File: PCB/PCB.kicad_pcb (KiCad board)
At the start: 2 copper layers, 121.6 x 80 mm, 109 parts, among them J2 Conn, J3 Screw_Terminal_01x02, J4 Screw_Terminal_01x02, J5 Screw_Terminal_01x02, J6 Screw_Terminal_01x02, Q1 Q_NPN_BCE, Q10 Q_NPN, Q11 Q_PNP_BCE, Q12 Q_NPN, Q13 Q_PNP, Q14 Q_PNP_BCE, Q15 Q_PNP_BCE, Q16 Q-NPN, Q17 Q-NPN, Q18 Q-NPN, Q19 Q-PNP, Q2 Q_PNP_BCE, Q20 Q-NPN, Q21 Q-PNP, Q22 Q-NPN, Q23 Q-PNP, Q24 Q-PNP, Q25 Q-NPN, Q26 Q-NPN, Q27 Q-PNP, Q28 Q-NPN, Q29 Q_PNP, Q3 Q_NPN_BCE, Q4 Q_PNP_BCE, Q5 Q_NPN_BCE, Q6 Q_PNP_BCE, Q7 Q_PNP_BCE, Q8 Q_NPN_BCE, Q9 Q_NPN_BCE

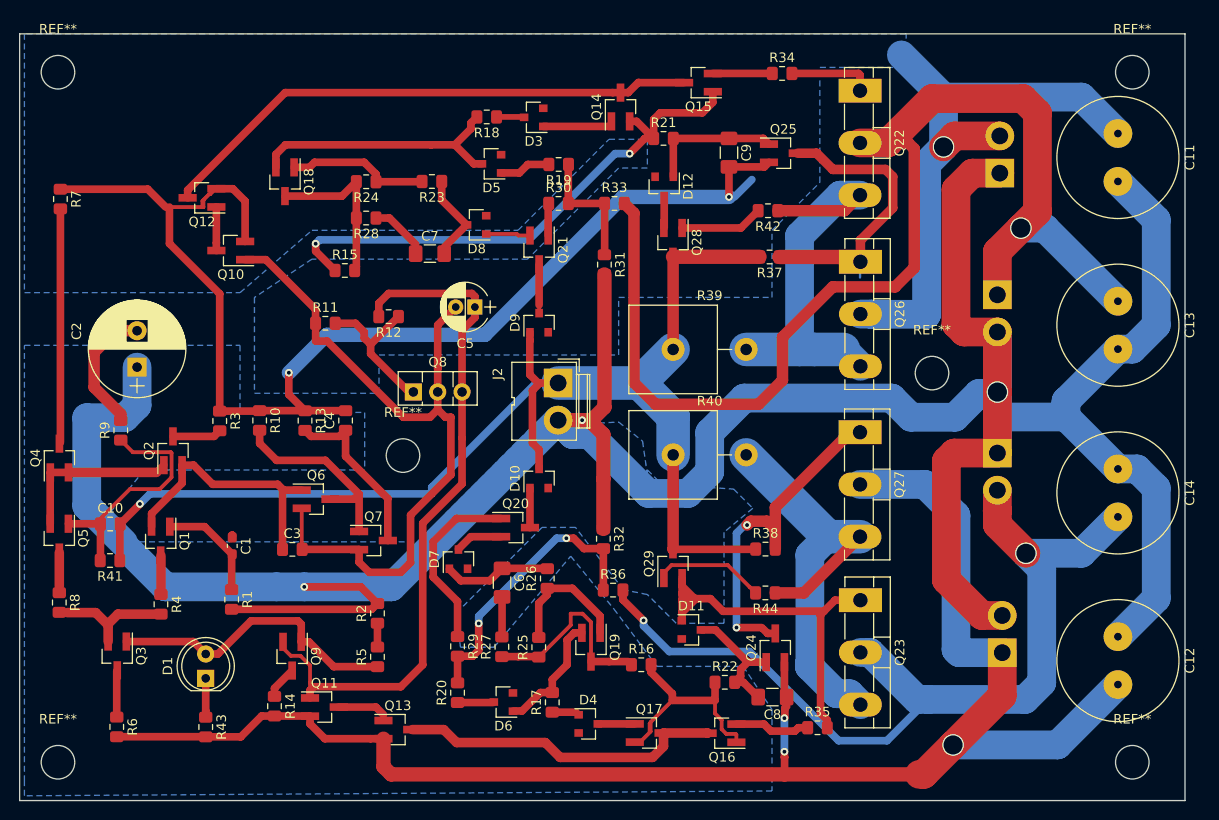
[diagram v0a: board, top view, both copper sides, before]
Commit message: rellené capas de abajo
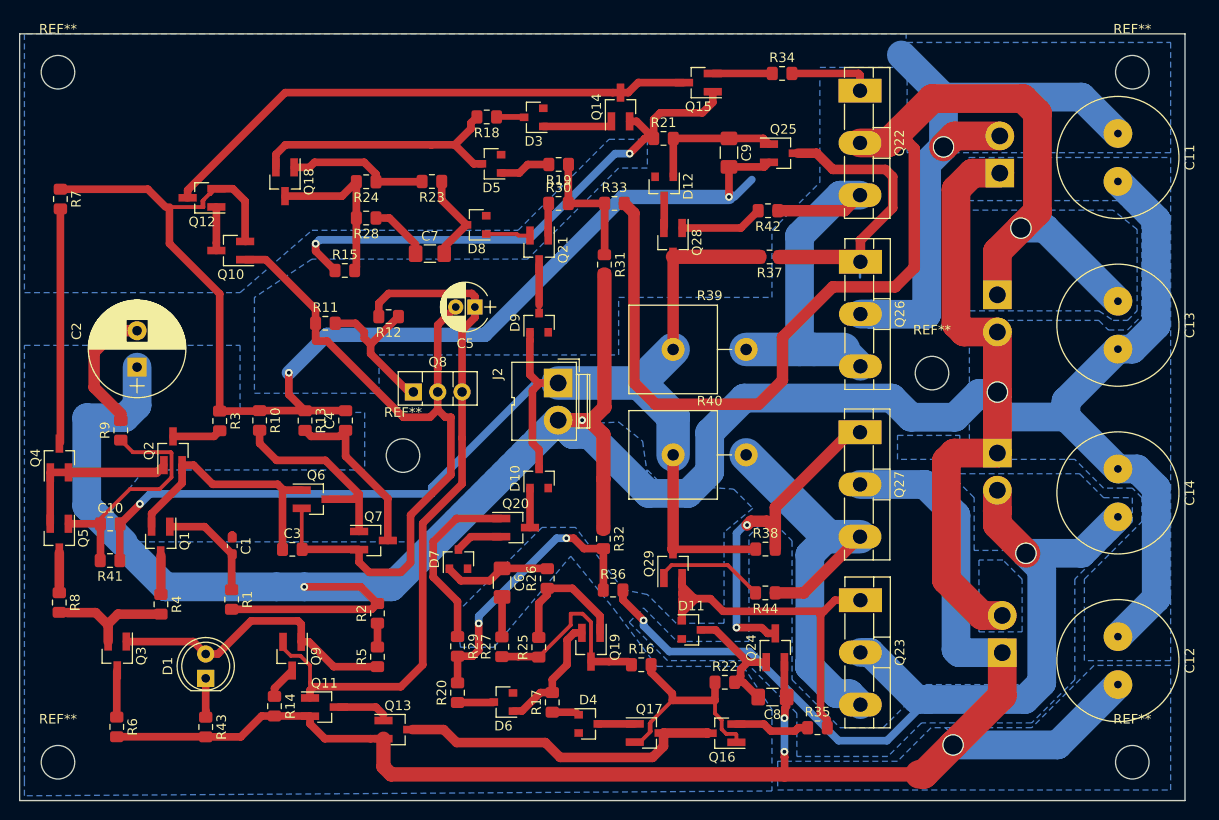
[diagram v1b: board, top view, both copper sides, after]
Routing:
- added copper zone on B.Cu, net +15V
- added copper zone on B.Cu, net -15V
- added copper zone on B.Cu, net VEE
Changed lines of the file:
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@@
-(kicad_pcb (version 20171130) (host pcbnew "(5.1.4)-1")
+(kicad_pcb (version 20171130) (host pcbnew "(5.1.2)-2")
   (general
     (thickness 1.6)
@@
   )
   (setup
-    (last_trace_width 0.8)
+    (last_trace_width 0.3)
     (user_trace_width 0.4)
     (user_trace_width 0.6)
@@
       )
     )
+  )
+  (zone (net 3) (net_name GND) (layer B.Cu) (hatch edge 0.508)
+    (connect_pads (clearance 0.508))
+    (min_thickness 0.254)
+    (fill yes (arc_segments 32) (thermal_gap 0.508) (thermal_bridge_width 0.508))
+    (polygon
+      (pts
+        (xy 254 64) (xy 255.5 62.5) (xy 276.5 62.5) (xy 276.5 115) (xy 267.5 115)
+        (xy 267.5 106.5) (xy 273.5 100.5) (xy 273.5 98) (xy 272.5 97) (xy 269.5 97)
+        (xy 266.5 94) (xy 255.5 94) (xy 255.5 79.5) (xy 269 79.5) (xy 270 80.5)
+        (xy 272 80.5) (xy 273.5 79) (xy 273.5 69.5) (xy 271 67) (xy 254 67)
+      )
+    )
+  )
+  (zone (net 58) (net_name -15V) (layer B.Cu) (hatch edge 0.508)
+    (connect_pads (clearance 0.508))
+    (min_thickness 0.254)
+    (fill yes (arc_segments 32) (thermal_gap 0.508) (thermal_bridge_width 0.508))
+    (polygon
+      (pts
+        (xy 248 91.5) (xy 254 91.5) (xy 254.5 91.5) (xy 254.5 95.5) (xy 267 95.5)
+        (xy 269.5 98) (xy 272.5 98) (xy 272.5 100.5) (xy 266.5 106.5) (xy 266.5 115.5)
+        (xy 266.5 117) (xy 262 121.5) (xy 250.5 121.5) (xy 247 125) (xy 237.5 125)
+        (xy 237.5 121) (xy 237.5 120.5) (xy 232 115) (xy 224 115) (xy 220 111)
+        (xy 221.5 109.5) (xy 225 113) (xy 232.5 113) (xy 232.5 102) (xy 234.5 100)
+        (xy 237 102.5) (xy 237 117) (xy 242 122) (xy 246.5 122) (xy 251 117.5)
+        (xy 261 117.5) (xy 262 116.5) (xy 262 106) (xy 259.5 103.5) (xy 256 103.5)
+        (xy 256 98) (xy 252 94) (xy 248 94)
+      )
+    )
+  )
+  (zone (net 3) (net_name GND) (layer B.Cu) (hatch edge 0.508)
+    (connect_pads (clearance 0.508))
+    (min_thickness 0.254)
+    (fill yes (arc_segments 32) (thermal_gap 0.508) (thermal_bridge_width 0.508))
+    (polygon
+      (pts
+        (xy 256.5 104.5) (xy 256.5 112) (xy 261 112) (xy 261 106.5) (xy 259 104.5)
+      )
+    )
+  )
+  (zone (net 14) (net_name VEE) (layer B.Cu) (hatch edge 0.508)
+    (connect_pads (clearance 0.508))
+    (min_thickness 0.254)
+    (fill yes (arc_segments 32) (thermal_gap 0.508) (thermal_bridge_width 0.508))
+    (polygon
+      (pts
+        (xy 253.5 122) (xy 251.5 122) (xy 248 125.5) (xy 235.5 125.5) (xy 235.5 128.5)
+        (xy 276.5 128.5) (xy 276.5 115.5) (xy 268.5 115.5) (xy 262 122) (xy 253 122)
+        (xy 255 124) (xy 255.5 124.5)
+      )
+    )
+  )
+  (zone (net 18) (net_name +15V) (layer B.Cu) (hatch edge 0.508)
+    (connect_pads (clearance 0.508))
+    (min_thickness 0.254)
+    (fill yes (arc_segments 32) (thermal_gap 0.508) (thermal_bridge_width 0.508))
+    (polygon
+      (pts
+        (xy 253.5 68) (xy 253.5 78.5) (xy 269 78.5) (xy 270.5 79.5) (xy 272 79.5)
+        (xy 273 78.5) (xy 273 70) (xy 270.5 68)
+      )
+    )
+  )
+  (zone (net 8) (net_name VCC) (layer B.Cu) (hatch edge 0.508)
+    (connect_pads (clearance 0.508))
+    (min_thickness 0.254)
+    (fill yes (arc_segments 32) (thermal_gap 0.508) (thermal_bridge_width 0.508))
+    (polygon
+      (pts
+        (xy 249 50.5) (xy 276.5 50.5) (xy 276.5 62) (xy 249 62)
+      )
+    )
